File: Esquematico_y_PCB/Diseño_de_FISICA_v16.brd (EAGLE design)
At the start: 100 x 78.7 mm, 40 parts, among them IC1 2133-DRV8825, IC2 2133-DRV8825, IC3 2133-DRV8825, J1 1X2-3.5MM, J3 1X2-3.5MM, Q1 BC817-25SMD

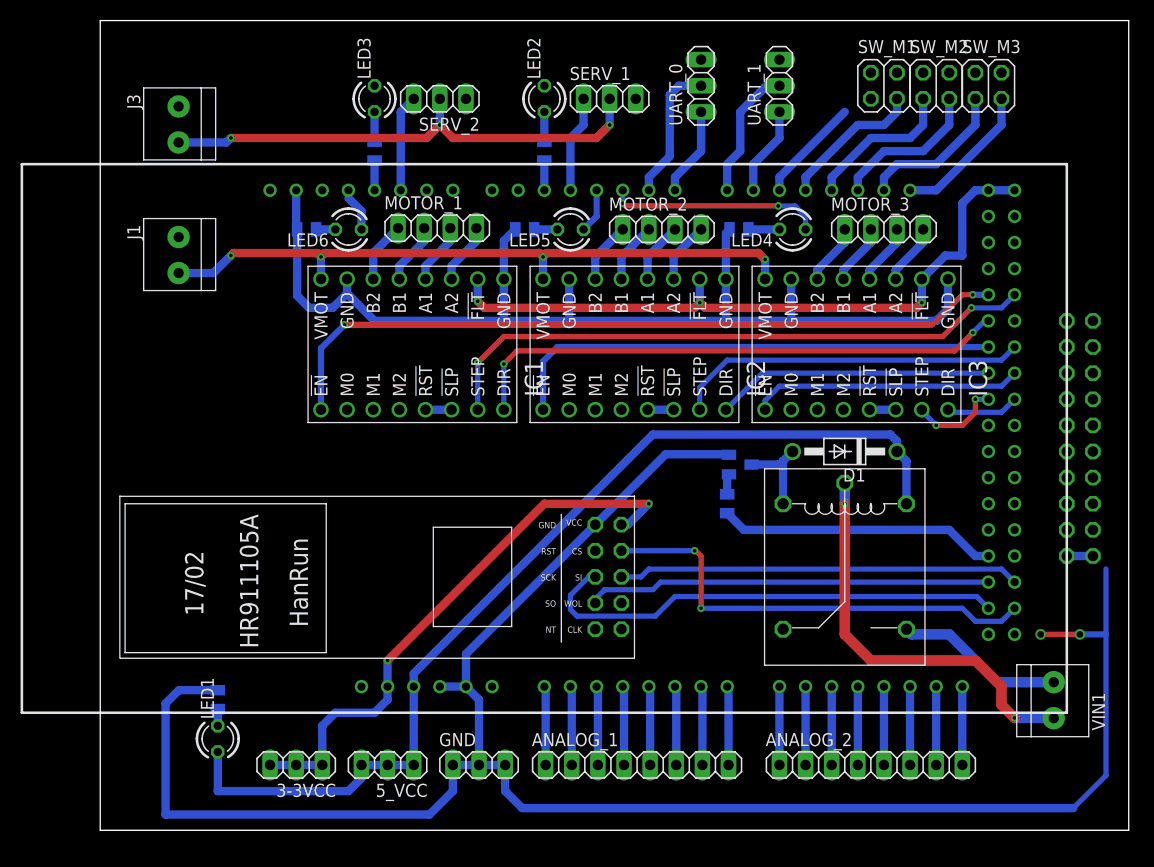
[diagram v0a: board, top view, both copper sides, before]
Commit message: Diseño PCB full
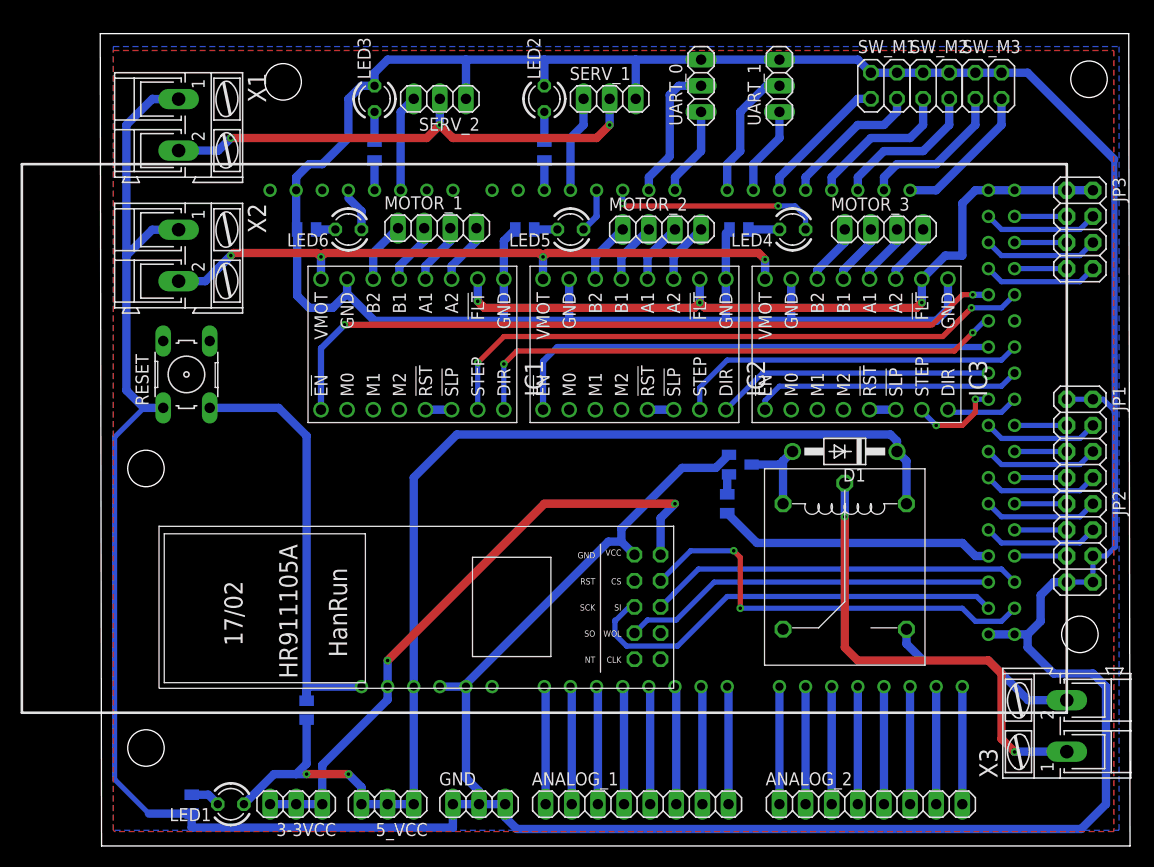
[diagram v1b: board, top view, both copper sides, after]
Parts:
- removed GPIO_DIG: (no value), pinhead:2X10
- removed J1, J3, VIN1: 1X2-3.5MM, adafruit:1X2-3.5MM
- added JP1, JP2, JP3: (no value), adafruit:2X04
- added R8: (no value), Resistor:RESC2012X65
- added RESET: (no value), switch-omron:B3F-10XX
- added X1, X2, X3: (no value), con-ptr500:AK300/2
- moved R1 10.5 mm to (8.89, 1.27), turned to 90 degrees
- moved LED1 6.48 mm to (12.7, 1.27), turned to 180 degrees
- moved MODULO_ETHERNET 4.80 mm to (55.8, 17.9)
- moved 3-3VCC 3.81 mm to (19.1, 1.27)
- moved 5_VCC 3.81 mm to (27.9, 1.27)
- moved ANALOG_1 3.81 mm to (52.2, 1.27)
- moved ANALOG_2 3.81 mm to (74.9, 1.27)
- moved GND 3.81 mm to (36.8, 1.27)
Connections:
- removed net D32: GPIO_DIG.1
- removed net D33: GPIO_DIG.2
- removed net D34: GPIO_DIG.3
- removed net D35: GPIO_DIG.4
- removed net D36: GPIO_DIG.5
- removed net D37: GPIO_DIG.6
- removed net D48: GPIO_DIG.17
- new net D22: ARDUINOMEGA2560.22, JP3.4
- new net D23: ARDUINOMEGA2560.23, JP3.3
- new net D24: ARDUINOMEGA2560.24, JP3.6
- new net D25: ARDUINOMEGA2560.25, JP3.5
- new net D26: ARDUINOMEGA2560.26, JP3.8
- new net D27: ARDUINOMEGA2560.27, JP3.7
- new net RESET: ARDUINOMEGA2560.RESET, R8.2, RESET.3
- net D38: now also JP1.4; no longer GPIO_DIG.7
- net D39: now also JP1.3; no longer GPIO_DIG.8
- net D40: now also JP1.6; no longer GPIO_DIG.9
- net D41: now also JP1.5; no longer GPIO_DIG.10
- net D42: now also ARDUINOMEGA2560.42, JP1.8; no longer GPIO_DIG.11
- net D43: now also ARDUINOMEGA2560.43, JP1.7; no longer GPIO_DIG.12
- net D44: now also ARDUINOMEGA2560.44, JP2.2; no longer GPIO_DIG.13
- net D45: now also ARDUINOMEGA2560.45, JP2.1; no longer GPIO_DIG.14
- net D46: now also ARDUINOMEGA2560.46, JP2.4; no longer GPIO_DIG.15
- net D47: now also ARDUINOMEGA2560.47, JP2.3; no longer GPIO_DIG.16
- net D49: now also JP2.5; no longer GPIO_DIG.18
- net GND: now also JP1.1, JP1.2, JP2.6, JP2.7, JP2.8, RESET.1, X1.1, X2.1; no longer GPIO_DIG.19, GPIO_DIG.20, J1.1, J3.1
- net N$1: now also X3.2; no longer VIN1.2
- net N$3: now also X3.1; no longer VIN1.1
- net VCC_5: now also JP3.1, JP3.2, R8.1
- net VCC_MOT: now also X2.2; no longer J1.2
- net VCC_SERVO: now also X1.2; no longer J3.2
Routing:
- net GND: track 299.6 -> 529.5 mm, vias 2 -> 0
- net RESET: track 0.00 -> 42.9 mm
- net VCC_5: track 163.3 -> 186.8 mm, vias 3 -> 5
- net D42: track 0.00 -> 11.2 mm
- net D40: track 0.00 -> 11.2 mm
- net D38: track 0.00 -> 11.2 mm
- net D26: track 0.00 -> 11.2 mm
- net D24: track 0.00 -> 11.2 mm
- net D22: track 0.00 -> 11.2 mm
- net D46: track 0.00 -> 11.2 mm
- net D44: track 0.00 -> 11.2 mm
- net VCC_3_3: track 55.3 -> 61.5 mm
- net N$3: track 39.4 -> 45.5 mm
- net D49: track 0.00 -> 5.08 mm
- net D47: track 0.00 -> 5.08 mm
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- added copper zone on layer 1, net GND
- added copper zone on layer 16, net GND
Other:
- board size 100 x 78.7 mm -> 100.1 x 79 mm
